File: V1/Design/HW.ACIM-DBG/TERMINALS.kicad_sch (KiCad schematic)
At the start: 20 parts, among them J3 SNAP PINOUT, J4 MICRO USB, J5 MCDBG PORT, Q2 MFET N, SW1 PRG SEL, U7 LOAD SWITCHER

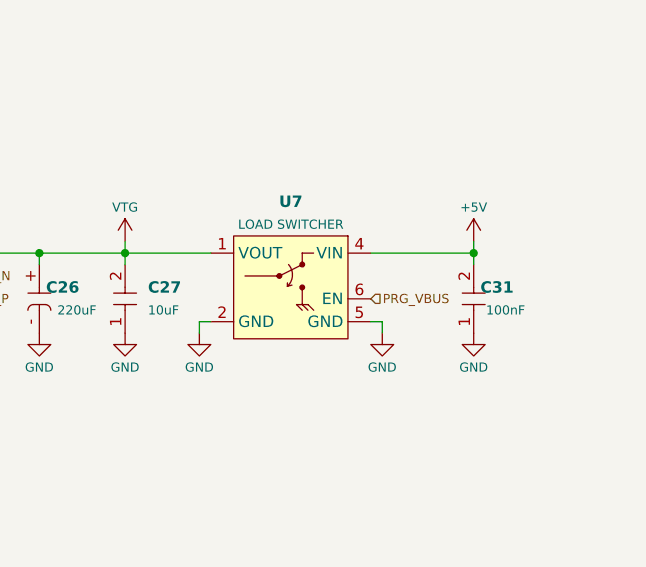
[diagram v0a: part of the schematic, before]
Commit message: V1 layout update 9
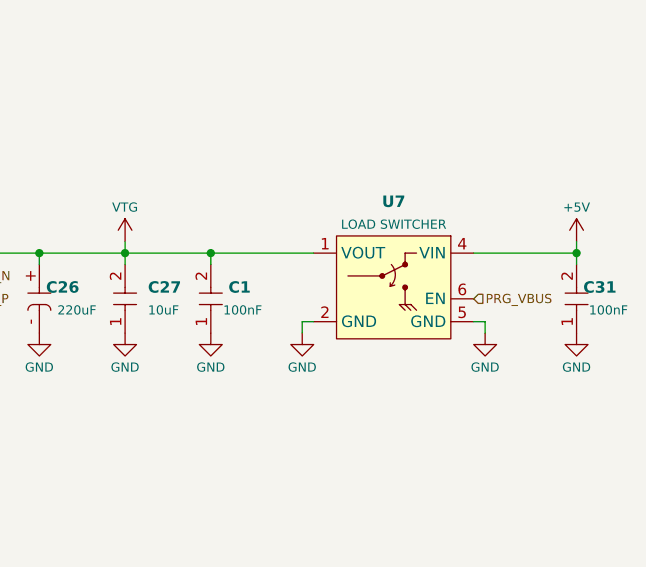
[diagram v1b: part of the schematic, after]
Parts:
- added C1: 100nF, SAMPI:CAP0603, symbol SAMPI:CERCAP
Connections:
- net GND: now also C1.1
- net VTG: now also C1.2
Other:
- moved on the sheet: C31, U7
